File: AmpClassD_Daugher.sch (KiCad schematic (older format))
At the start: 81 parts, among them J1 POWER, J10 MONO, J11 LEFT, J12 PLIM_DEF, J13 OUTS, J14 INS, J15 PWR, J16 GND, J17 R+, J18 L+, J2 POWER, J3 AUDIO_IN, J4 ST/MN, J5 GAIN_DEF, J6 SYNC_DEFAULT, J7 MN, J8 MN, J9 RIGHT, Q1 MMBT3904, Q2 MMBT3904, Q3 MMBT3904, Q4 MMBT3904, Q5 MMBT3904, U1 NE5532, U2 NE5532, U3 TPA3118D2

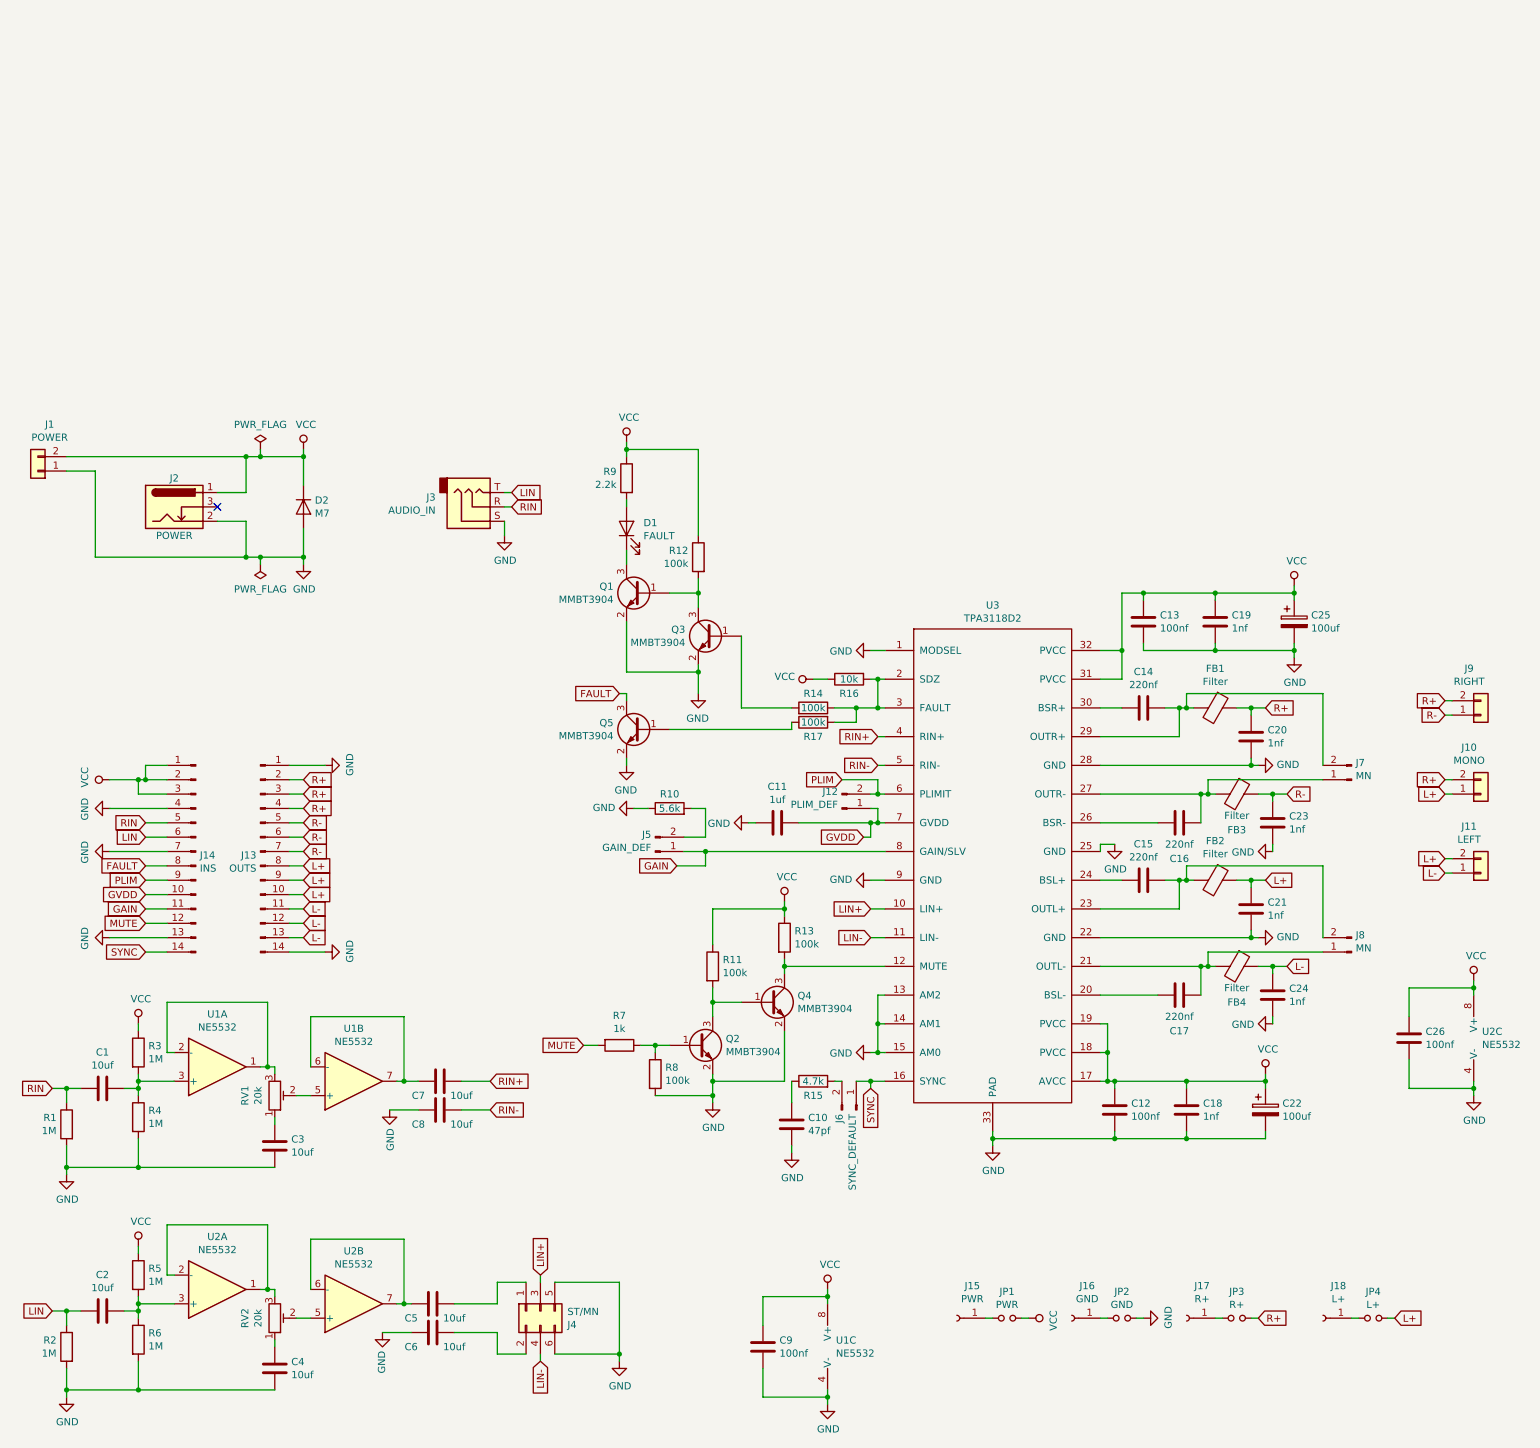
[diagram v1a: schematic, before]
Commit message: updated schematic
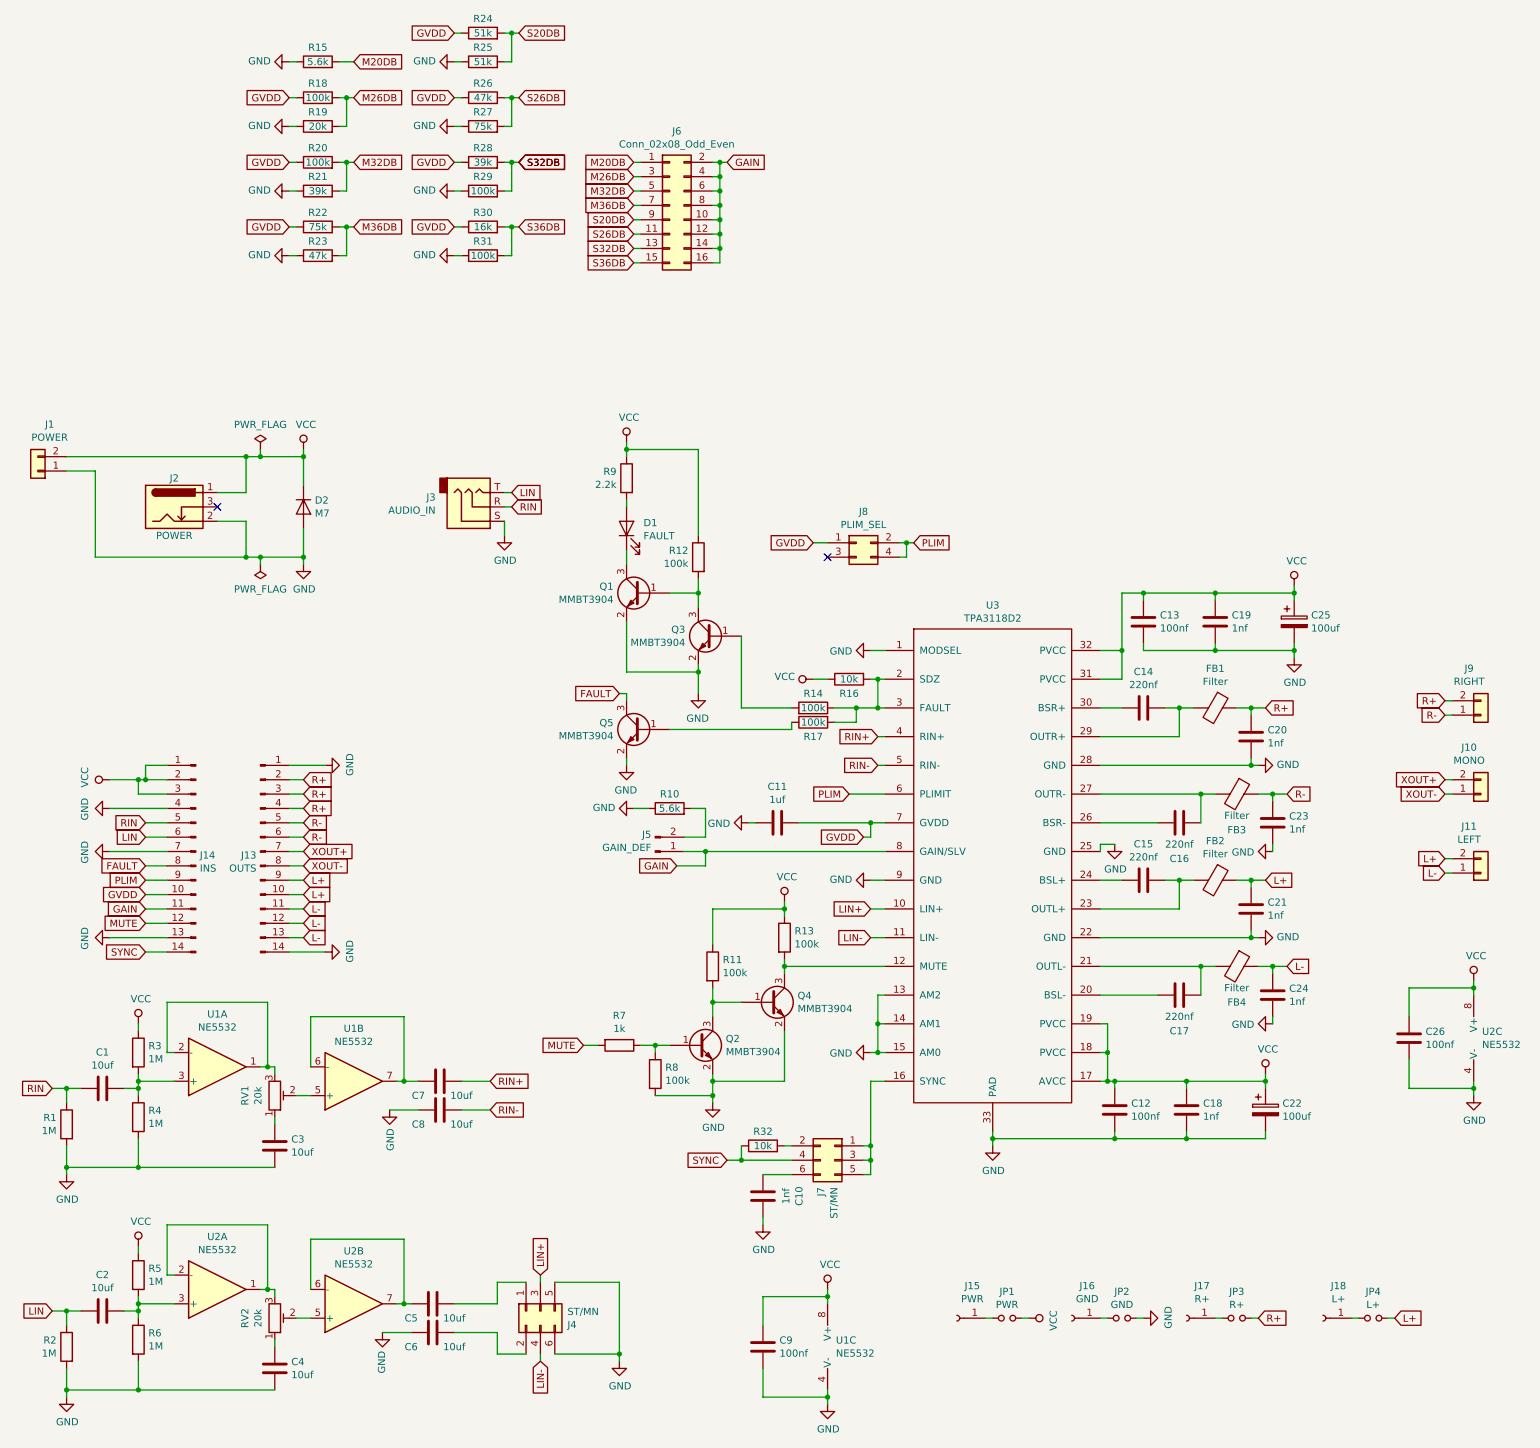
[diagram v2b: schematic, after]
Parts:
- removed J12: PLIM_DEF, Connector_PinHeader_2.54mm:PinHeader_1x02_P2.54mm_Vertical_SMD_Pin1Right, symbol Connector:Conn_01x02_Male
- removed J6: SYNC_DEFAULT, Connector_PinHeader_2.54mm:PinHeader_1x02_P2.54mm_Vertical_SMD_Pin1Right, symbol Connector:Conn_01x02_Male
- removed J7, J8: MN, Connector_PinHeader_2.54mm:PinHeader_1x02_P2.54mm_Vertical_SMD_Pin1Right, symbol Connector:Conn_01x02_Male
- added J6: Conn_02x08_Odd_Even, symbol Connector_Generic:Conn_02x08_Odd_Even
- added J7: ST/MN, Connector_PinHeader_2.54mm:PinHeader_2x03_P2.54mm_Vertical_SMD, symbol Connector_Generic:Conn_02x03_Odd_Even
- added J8: PLIM_SEL, symbol Connector_Generic:Conn_02x02_Odd_Even
- added R18, R20, R29, R31: 100k, Resistor_SMD:R_0603_1608Metric_Pad1.05x0.95mm_HandSolder_SmallRef, symbol Device:R
- added R19: 20k, Resistor_SMD:R_0603_1608Metric_Pad1.05x0.95mm_HandSolder_SmallRef, symbol Device:R
- added R21, R28: 39k, Resistor_SMD:R_0603_1608Metric_Pad1.05x0.95mm_HandSolder_SmallRef, symbol Device:R
- added R22, R27: 75k, Resistor_SMD:R_0603_1608Metric_Pad1.05x0.95mm_HandSolder_SmallRef, symbol Device:R
- added R23, R26: 47k, Resistor_SMD:R_0603_1608Metric_Pad1.05x0.95mm_HandSolder_SmallRef, symbol Device:R
- added R24, R25: 51k, Resistor_SMD:R_0603_1608Metric_Pad1.05x0.95mm_HandSolder_SmallRef, symbol Device:R
- added R30: 16k, Resistor_SMD:R_0603_1608Metric_Pad1.05x0.95mm_HandSolder_SmallRef, symbol Device:R
- added R32: 10k, Resistor_SMD:R_0603_1608Metric_Pad1.05x0.95mm_HandSolder_SmallRef, symbol Device:R
- C10: value 47pf -> 1nf
- R15: value 4.7k -> 5.6k
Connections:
- net GAIN: now also J6.10 (Pin_10), J6.12 (Pin_12), J6.14 (Pin_14), J6.16 (Pin_16), J6.2 (Pin_2), J6.4 (Pin_4), J6.6 (Pin_6), J6.8 (Pin_8)
- net GND: now also C10.1, R15.1, R19.1, R21.1, R23.1, R25.1, R27.1, R29.1, R31.1; no longer C10.2
- net GVDD: now also J8.1 (Pin_1), R18.1, R20.1, R22.1, R24.1, R26.1, R28.1, R30.1
- net L+: no longer J10.1 (Pin_1), J13.8 (Pin_8)
- net PLIM: now also J8.2 (Pin_2), J8.4 (Pin_4)
- net R+: no longer J10.2 (Pin_2)
- net R-: no longer J13.7 (Pin_7)
- net SYNC: now also J7.4 (Pin_4), R32.1; no longer U3.16 (SYNC)
- net M20DB: now reaches R15.2
- net M20DB: now also J6.1 (Pin_1)
- new net: J7.1 (Pin_1), J7.3 (Pin_3), J7.5 (Pin_5), U3.16 (SYNC)
- new net: J7.2 (Pin_2), R32.2
- new net: C10.2, J7.6 (Pin_6)
- new net M26DB: J6.3 (Pin_3), R18.2, R19.2
- new net M32DB: J6.5 (Pin_5), R20.2, R21.2
- new net M36DB: J6.7 (Pin_7), R22.2, R23.2
- new net S20DB: J6.9 (Pin_9), R24.2, R25.2
- new net S26DB: J6.11 (Pin_11), R26.2, R27.2
- new net S32DB: J6.13 (Pin_13), R28.2, R29.2
- new net S36DB: J6.15 (Pin_15), R30.2, R31.2
- new net XOUT+: J10.2 (Pin_2), J13.7 (Pin_7)
- new net XOUT-: J10.1 (Pin_1), J13.8 (Pin_8)
- no-connect marks 1 -> 2
